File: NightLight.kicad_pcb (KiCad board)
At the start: 2 copper layers, 88 x 88 mm, 17 parts, among them U1 magnetic-charger, U2 rdm-6300, U3 TP4056, U4 ESP32-WROOM-32

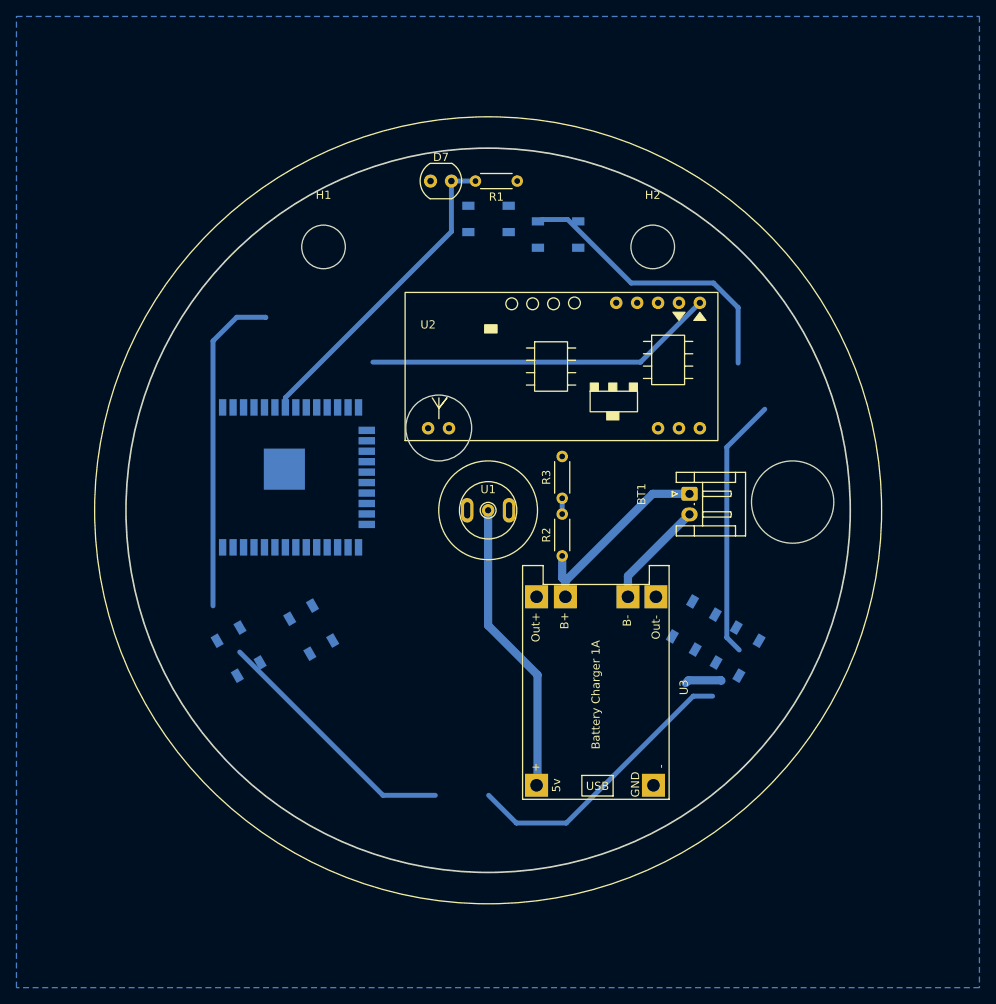
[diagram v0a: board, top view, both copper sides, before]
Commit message: Add lots of ocmponents
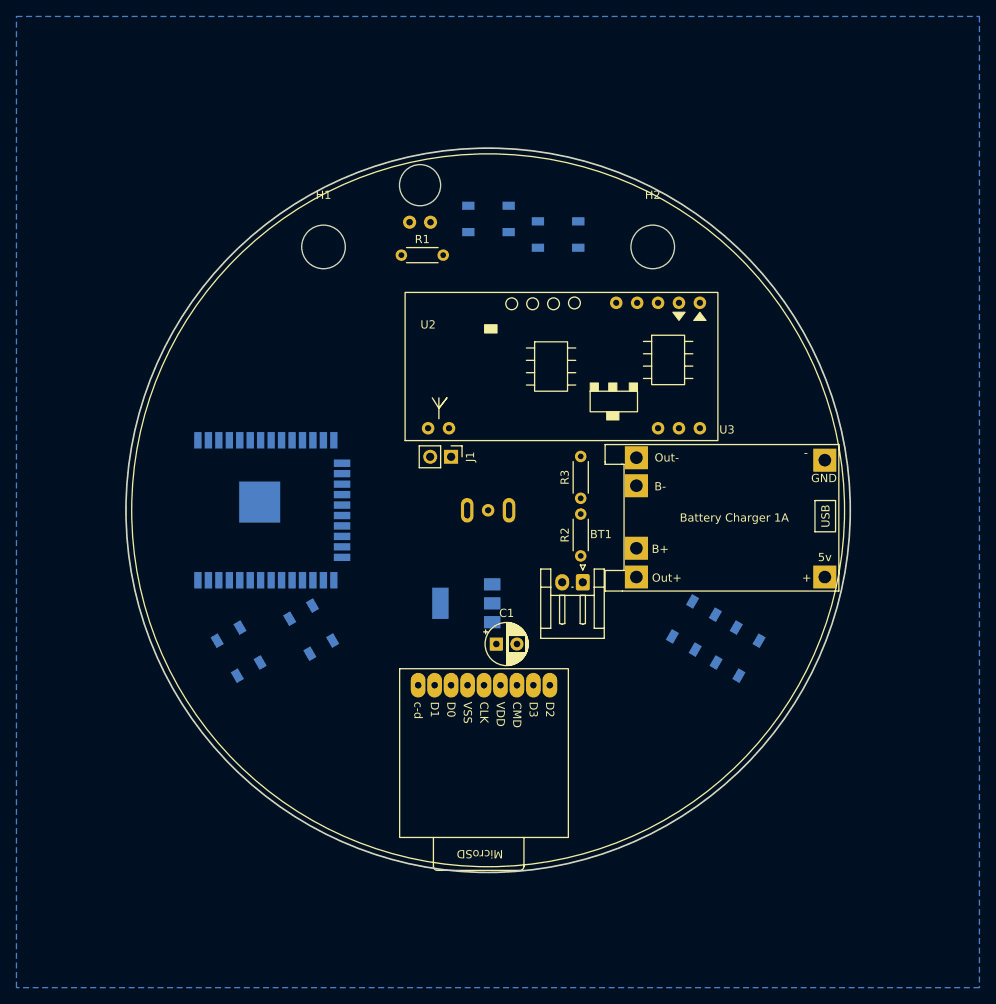
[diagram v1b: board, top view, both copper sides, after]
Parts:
- added C1: 22u, Capacitor_THT:CP_Radial_D5.0mm_P2.50mm, F.Cu at (101.0, 116.2)
- added J1: Conn_01x02, Connector_PinHeader_2.54mm:PinHeader_1x02_P2.54mm_Vertical, F.Cu at (95.5, 93.5)
- added J2: Micro_SD_Card, sd-card:sd-card, F.Cu at (99.5, 121.2)
- added U5: AMS1117-3.3, Package_TO_SOT_SMD:SOT-223-3_TabPin2, B.Cu at (97.3, 111.3)
- D7, U1: moved to B.Cu
- moved U3 46.0 mm to (142.6, 109.8), turned to 180 degrees
- moved BT1 16.8 mm to (111.5, 108.8), turned to 180 degrees
- moved R1 16.7 mm to (89.5, 69.0), turned to 0 degrees
- moved D7 5.00 mm to (93.0, 65.0), turned to 180 degrees
- moved U4 5.00 mm to (73.0, 100.0)
- moved R2 2.25 mm to (111.2, 105.5)
- moved R3 2.25 mm to (111.2, 98.5)
- turned U1 to 180 degrees
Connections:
- U2 pad 6: unconnected-(U2-Pad6) -> Net-(J1-Pad1)
- U2 pad 7: unconnected-(U2-Pad7) -> Net-(J1-Pad2)
- U3 pad 3: +3V3 -> +4V
- U4 pad 10: unconnected-(U4-Pad10) -> DAC1
- U4 pad 11: unconnected-(U4-Pad11) -> DAC2
- U4 pad 12: unconnected-(U4-Pad12) -> TOUCH3
- U4 pad 8: unconnected-(U4-Pad8) -> TOUCH1
- U4 pad 9: unconnected-(U4-Pad9) -> TOUCH2
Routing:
- net Net-(D5-Pad1): track 70.8 -> 0.00 mm
- net unconnected-(U2-Pad4): track 42.7 -> 0.00 mm
- net PHOTO_VOLTAGE: track 38.8 -> 0.00 mm
- net GND: track 36.3 -> 0.00 mm
- net +5V: track 35.9 -> 0.00 mm
- net +3V3: track 35.1 -> 0.00 mm
- net Net-(D2-Pad1): track 35.0 -> 0.00 mm
- net +BATT: track 24.6 -> 0.00 mm
- net -BATT: track 13.1 -> 0.00 mm
- net ADC_BAT: track 1.92 -> 0.00 mm
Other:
- outline, holes or cut-outs redrawn
- board text added: "TODO: - Batterie ausmessen - Speaker Optionen auschecken - How far does the SD card protrude"
